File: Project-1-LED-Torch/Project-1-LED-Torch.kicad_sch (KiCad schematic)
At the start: 4 parts, among them SW1 SW_DPDT_x2

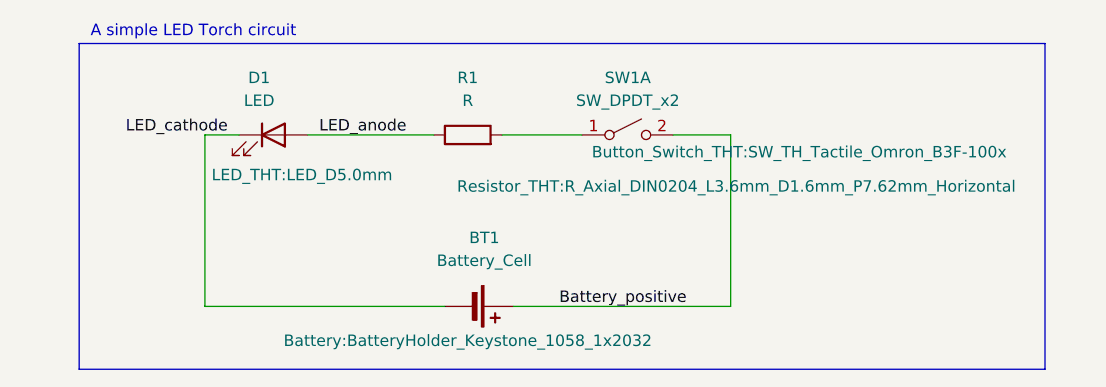
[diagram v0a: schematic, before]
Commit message: do schematic design, step 7, add comments inc footprints notes
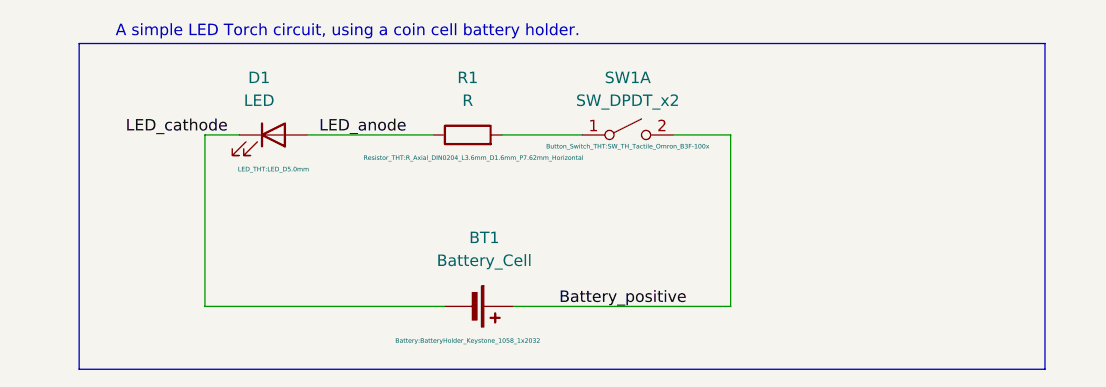
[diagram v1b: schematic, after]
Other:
- note added: "A simple LED Torch circuit, using a coin cell battery holder."
- note removed: "A simple LED Torch circuit"
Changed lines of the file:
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@@
 		)
 	)
-	(text "A simple LED Torch circuit"
-		(exclude_from_sim no)
-		(at 100.33 64.77 0)
+	(text "A simple LED Torch circuit, using a coin cell battery holder."
+		(exclude_from_sim no)
+		(at 117.475 64.77 0)
 		(effects
 			(font
@@
 		)
 		(property "Footprint" "Resistor_THT:R_Axial_DIN0204_L3.6mm_D1.6mm_P7.62mm_Horizontal"
-			(at 160.655 81.915 90)
-			(show_name no)
-			(do_not_autoplace no)
-			(effects
-				(font
-					(size 1.27 1.27)
+			(at 131.445 78.74 90)
+			(show_name no)
+			(do_not_autoplace no)
+			(effects
+				(font
+					(size 0.5 0.5)
 				)
 			)
@@
 		)
 		(property "Footprint" "LED_THT:LED_D5.0mm"
-			(at 112.395 80.645 0)
-			(show_name no)
-			(do_not_autoplace no)
-			(effects
-				(font
-					(size 1.27 1.27)
+			(at 109.22 80.01 0)
+			(show_name no)
+			(do_not_autoplace no)
+			(effects
+				(font
+					(size 0.5 0.5)
 				)
 			)
@@
 		)
 		(property "Footprint" "Button_Switch_THT:SW_TH_Tactile_Omron_B3F-100x"
-			(at 167.64 78.105 0)
-			(show_name no)
-			(do_not_autoplace no)
-			(effects
-				(font
-					(size 1.27 1.27)
+			(at 148.59 77.47 0)
+			(show_name no)
+			(do_not_autoplace no)
+			(effects
+				(font
+					(size 0.5 0.5)
 				)
 			)
@@
 			(effects
 				(font
-					(size 1.27 1.27)
-				)
-			)
+					(size 0.5 0.5)
+				)
+			)
